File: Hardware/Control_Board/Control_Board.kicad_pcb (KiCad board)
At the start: 2 copper layers, 129.5 x 130.8 mm, 47 parts, among them J1 Raspberry_Pi_2_3, J112 19705-4301, J2 Screw_Terminal_01x02, J3 Screw_Terminal_01x02, J4 19705-4301, J5 19705-4301, J6 19705-4301, J8 19705-4301, K1 ALQ3F12, K2 ALQ3F12, K3 ALQ3F12, K4 ALQ3F12, Q1 PMOS, Q2 Q_Dual_PMOS_S1G1S2G2D2D2D1D1, U1 ULN2003, U2 ULN2003, U3 TPS563200

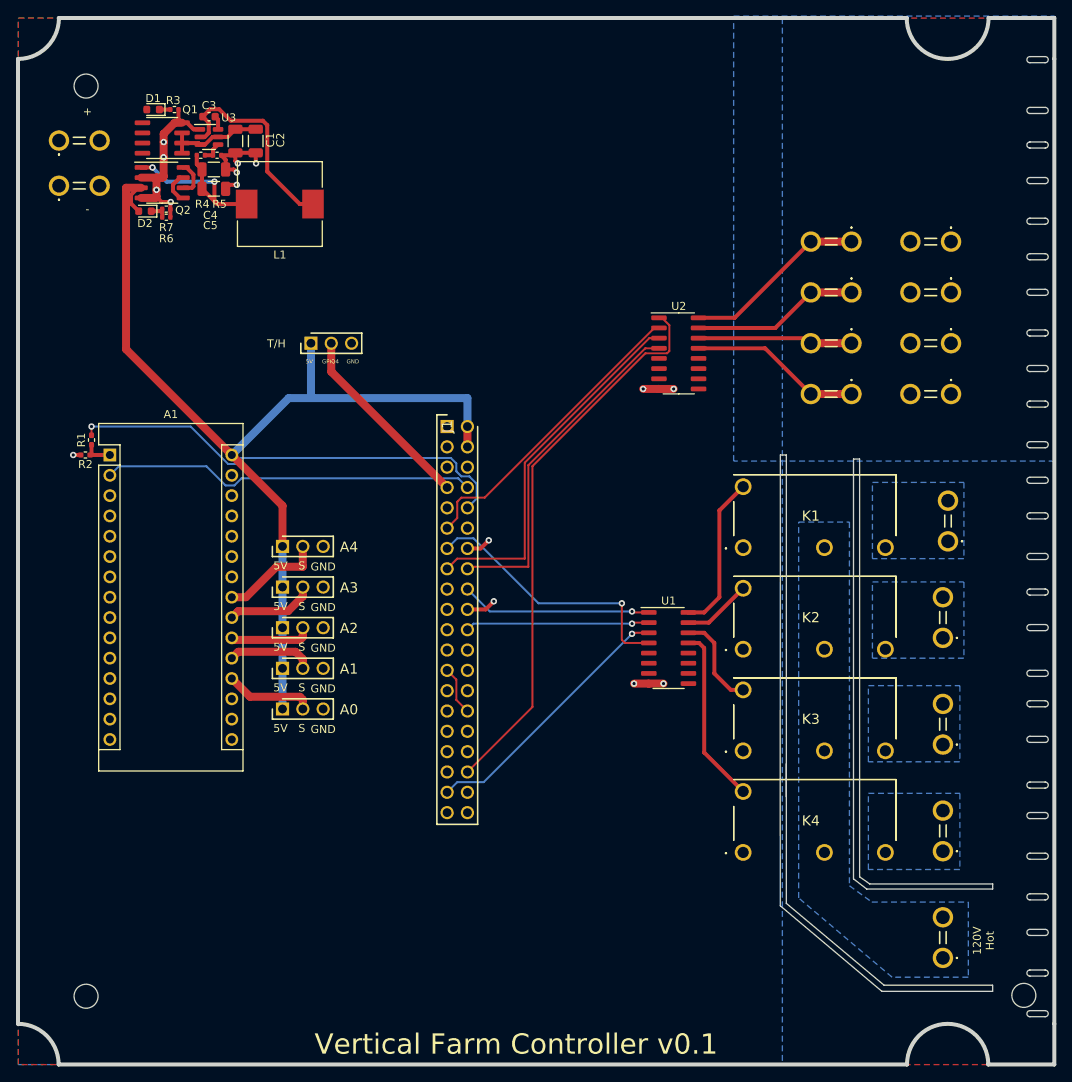
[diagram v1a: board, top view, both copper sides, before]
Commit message: Update Control_Board.kicad_pcb
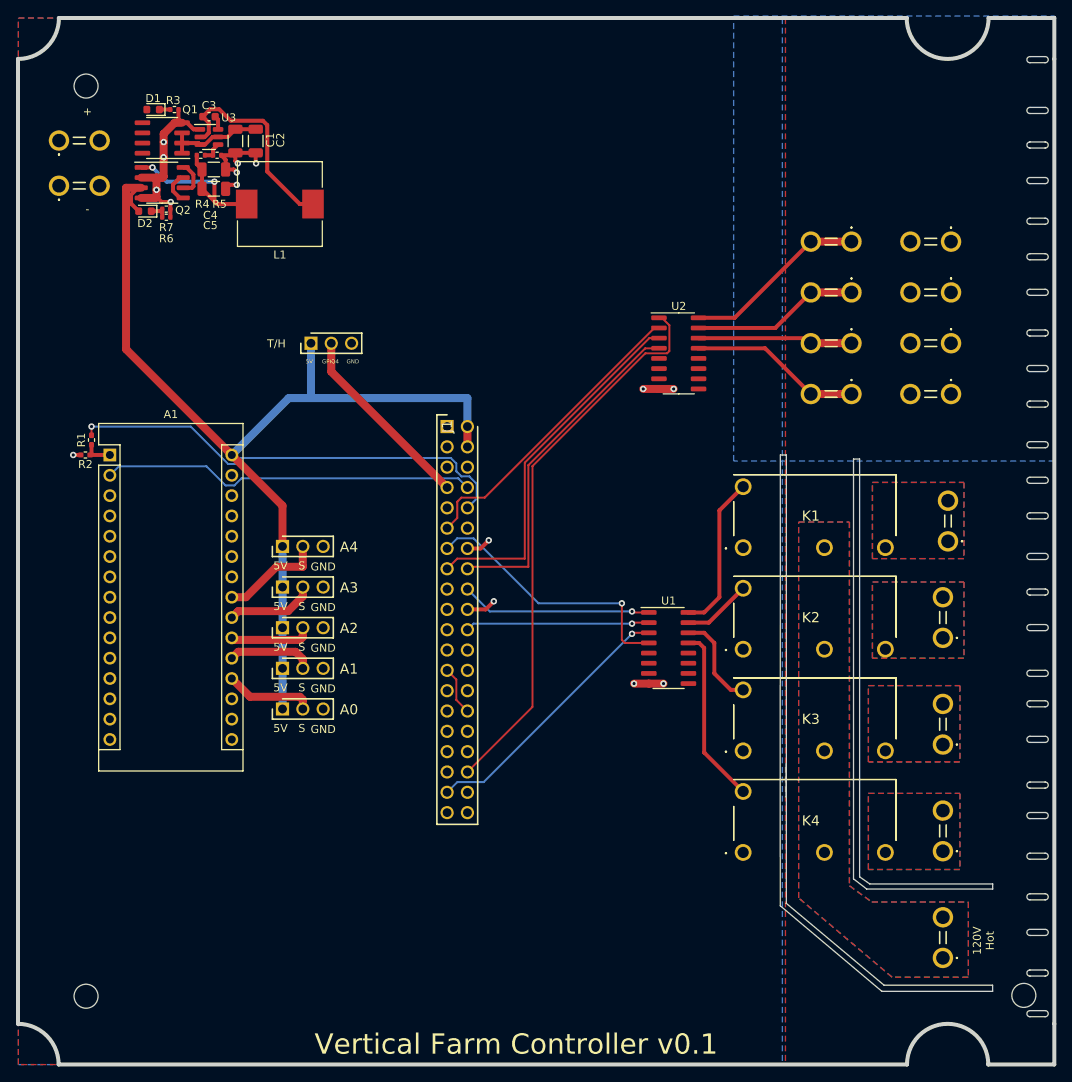
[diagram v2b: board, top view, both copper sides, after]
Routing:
- added copper zone on F.Cu, net 120V_Hot
- added copper zone on F.Cu, net Net-(K1-Pad3)
- added copper zone on F.Cu, net Net-(K2-Pad3)
- added copper zone on F.Cu, net Net-(K3-Pad3)
- added copper zone on F.Cu, net Net-(K4-Pad3)
